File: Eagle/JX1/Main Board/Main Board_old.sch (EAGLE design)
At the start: 10 parts, among them U1 SN74HC595N, U2 SN74HC595N

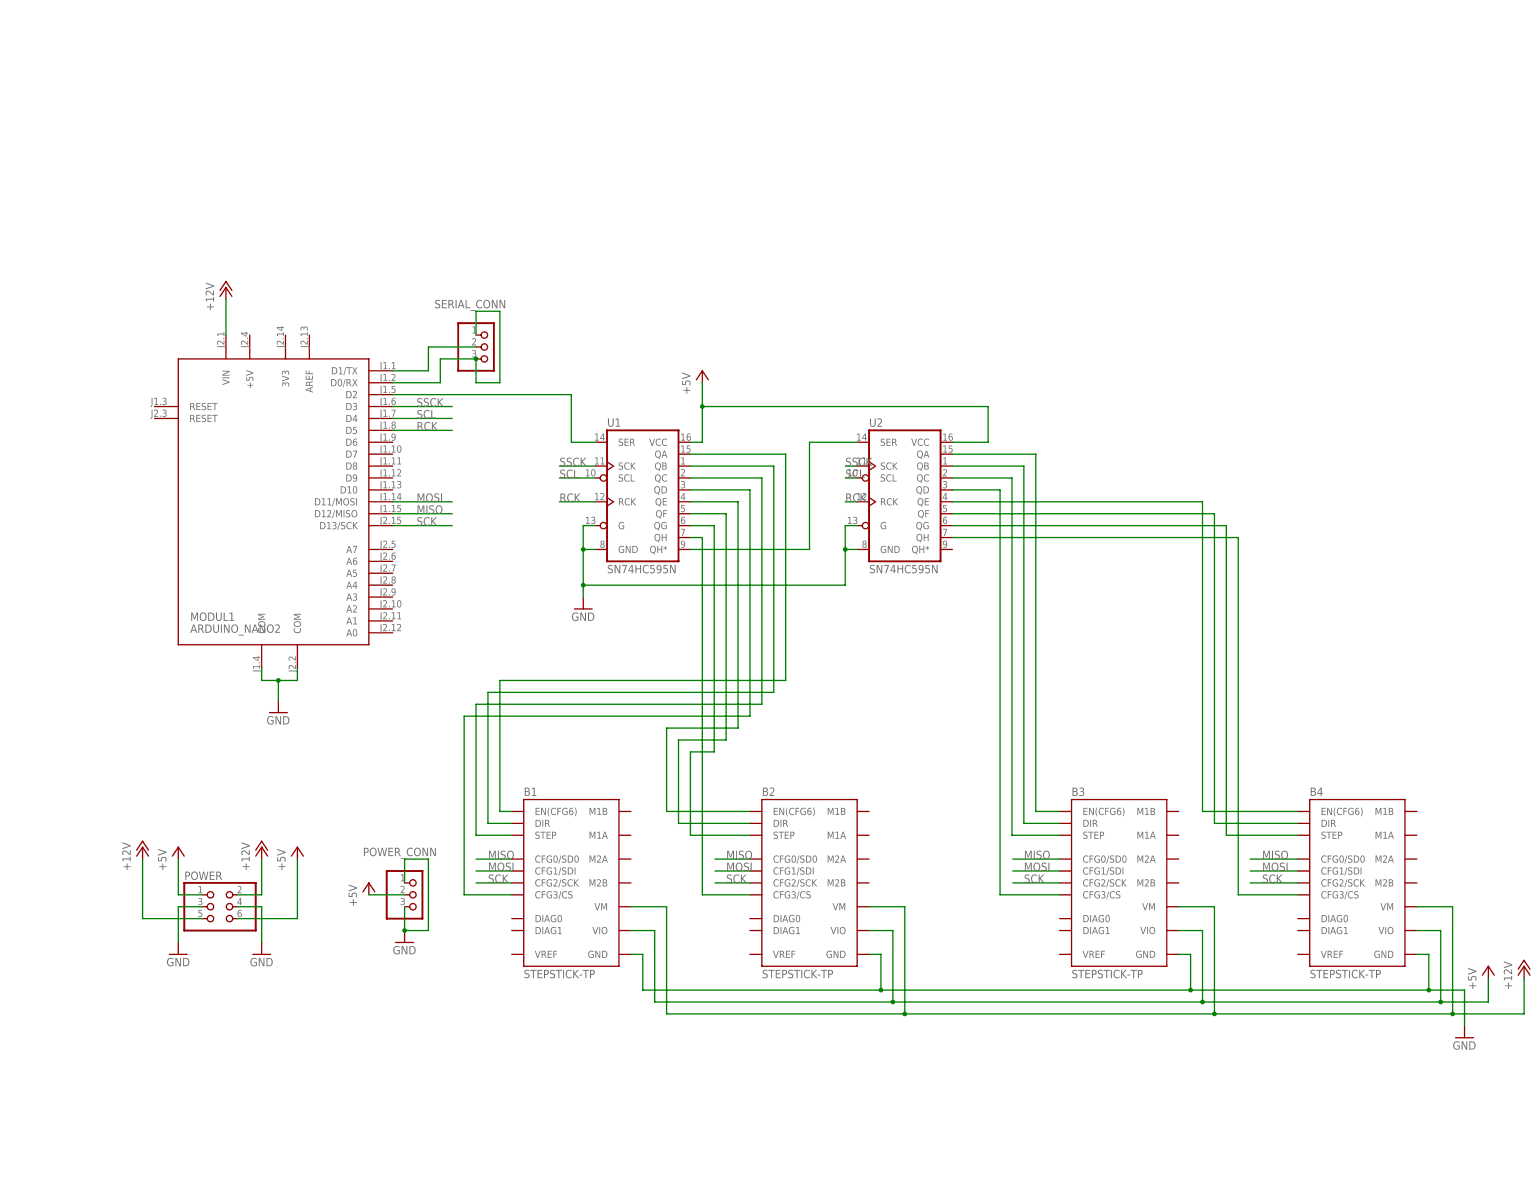
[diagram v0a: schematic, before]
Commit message: More board Changes
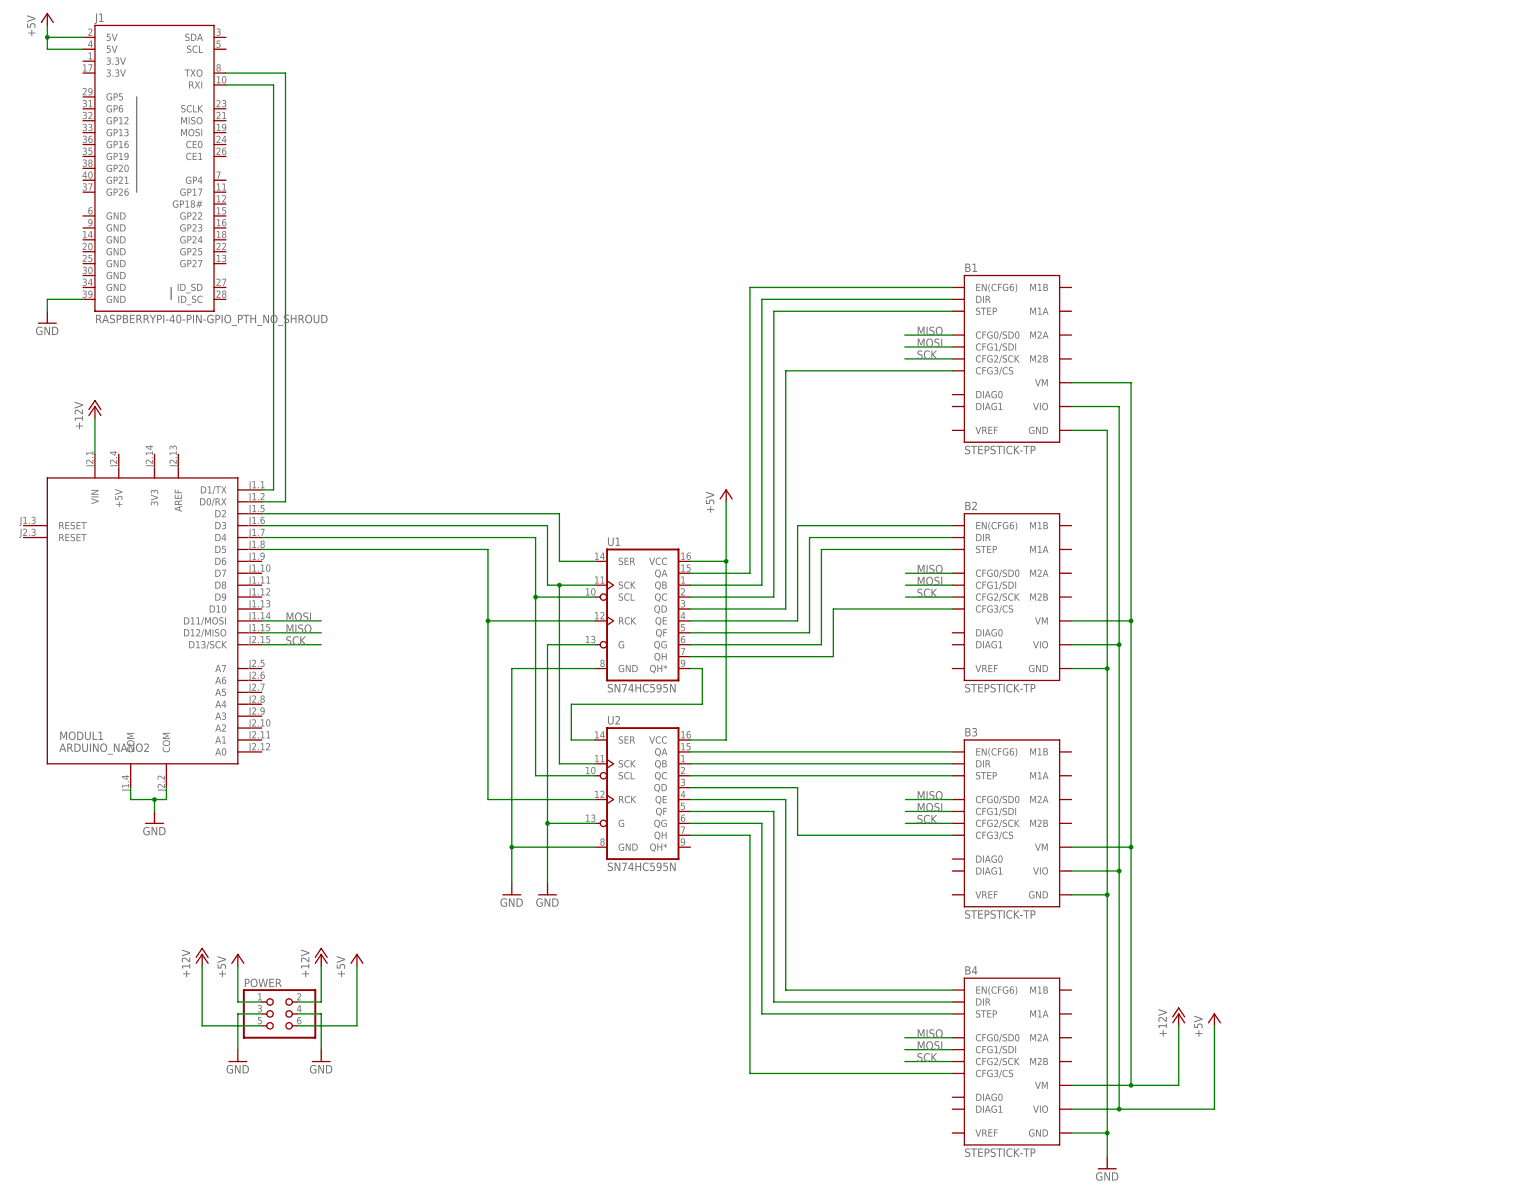
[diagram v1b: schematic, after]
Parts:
- removed POWER_CONN, SERIAL_CONN: (no value), pinhead:PINHD-1X3
- added J1: RASPBERRYPI-40-PIN-GPIO_PTH_NO_SHROUD, SparkFun-Connectors:RASPBERRYPI-40-PIN-GPIO_PTH_NO_SHROUD
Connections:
- net RCK renamed N$25
- net SCL renamed N$24
- net SSCK renamed N$23
- removed net N$1: MODUL1.D1/TX, SERIAL_CONN.2
- new net N$26: J1.RXI, MODUL1.D1/TX
- net +5V: now also J1.5V@2, J1.5V@4; no longer POWER_CONN.2
- net GND: now also J1.GND@39; no longer POWER_CONN.1, POWER_CONN.3
- net N$27: now also J1.TXO; no longer SERIAL_CONN.1, SERIAL_CONN.3
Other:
- moved on the sheet: B1, B2, B3, B4, MODUL1, POWER, U1, U2
